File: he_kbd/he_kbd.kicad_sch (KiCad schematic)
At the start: 270 parts, among them J1 AudioJack4, J2 Conn_01x08_Pin, J3 AudioJack4, J4 Conn_01x08_Pin

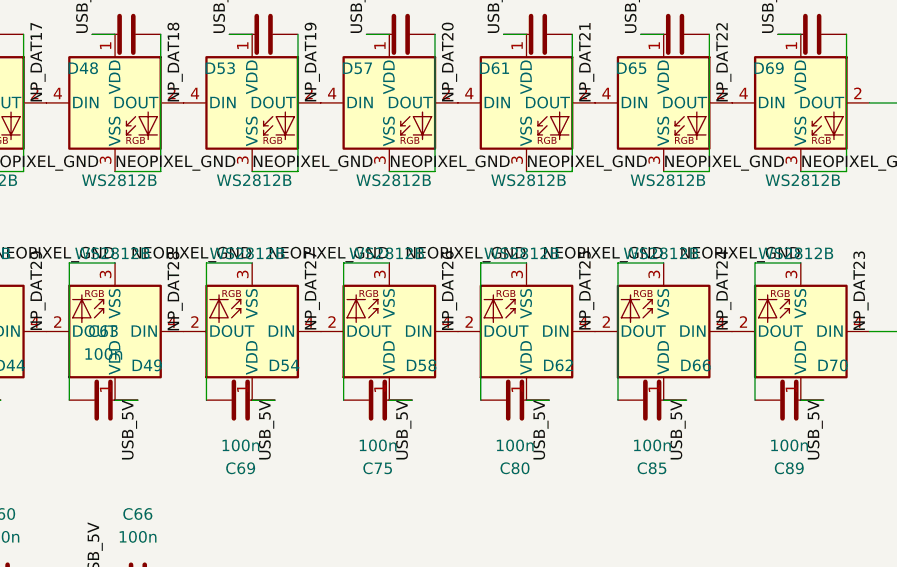
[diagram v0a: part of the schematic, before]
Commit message: so far so good
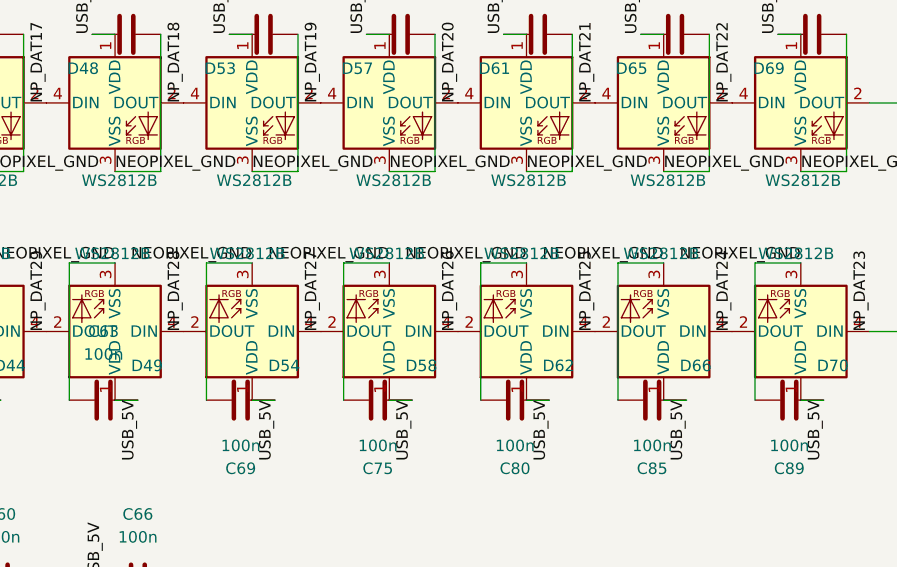
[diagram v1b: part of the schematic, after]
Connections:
- net NP_DAT24: now also D66.4 (DIN), D70.2 (DOUT)
- net NP_DAT25: now also D62.4 (DIN), D66.2 (DOUT)
- net NP_DAT27: now also D54.4 (DIN), D58.2 (DOUT)
- net NP_DAT28: now also D49.4 (DIN), D54.2 (DOUT)
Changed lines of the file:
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@@
 	)
 	(label "NP_DAT25"
-		(at 524.51 271.7316 90)
+		(at 524.51 271.78 90)
 		(effects
 			(font
@@
 	)
 	(label "NP_DAT27"
-		(at 494.03 271.7316 90)
+		(at 494.03 271.78 90)
 		(effects
 			(font
@@
 	)
 	(label "NP_DAT24"
-		(at 539.75 271.7316 90)
+		(at 539.75 271.78 90)
 		(effects
 			(font
@@
 	)
 	(label "NP_DAT28"
-		(at 478.79 271.8222 90)
+		(at 478.79 271.78 90)
 		(effects
 			(font
